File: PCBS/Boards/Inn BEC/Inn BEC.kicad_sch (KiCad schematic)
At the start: 7 parts, among them J1 Conn_01x02_Pin, J2 Conn_01x02_Pin, U1 XL1509-5.0

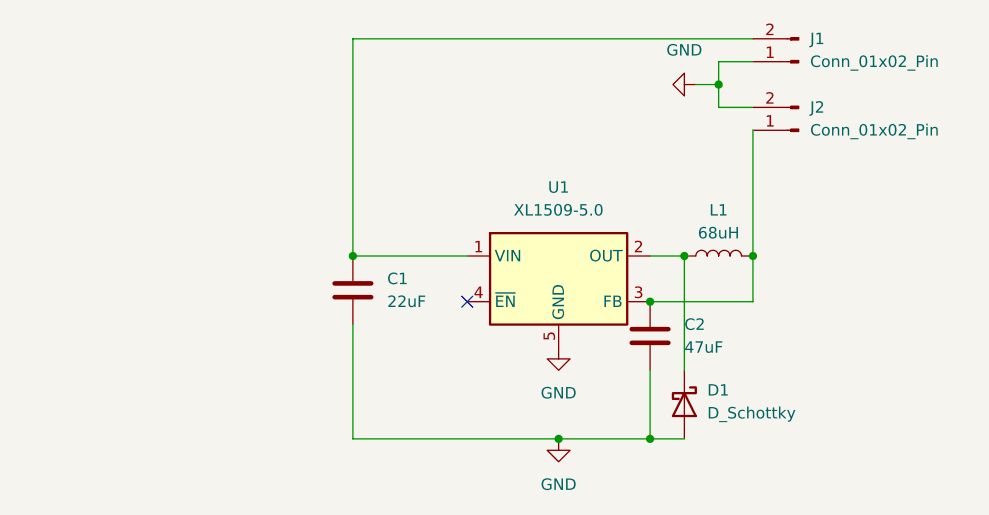
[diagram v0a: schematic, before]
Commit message: created SHU BEC, added KiCad project files and production files
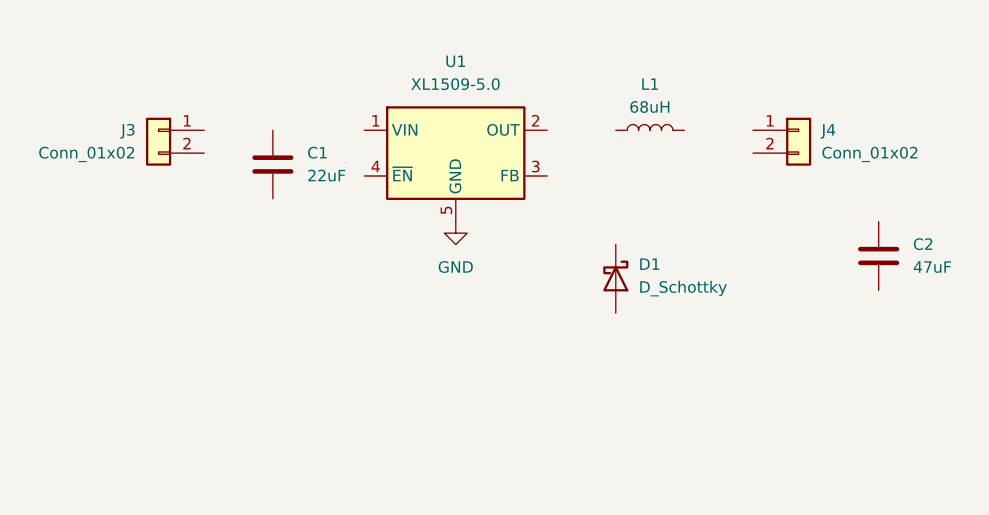
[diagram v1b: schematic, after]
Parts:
- removed J1, J2: Conn_01x02_Pin, Connector_Wire:SolderWire-0.1sqmm_1x02_P3.6mm_D0.4mm_OD1mm, symbol Connector:Conn_01x02_Pin
- added J3, J4: Conn_01x02, symbol Connector_Generic:Conn_01x02
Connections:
- net GND: no longer C1.2, C2.2, D1.2 (A)
- net at U1.1 (VIN): no longer C1.1
- now unconnected: C2.1, D1.1 (K), L1.1, L1.2, U1.2 (OUT), U1.3 (FB)
- no-connect marks 1 -> 0
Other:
- moved on the sheet: C1, C2, D1, L1, U1
